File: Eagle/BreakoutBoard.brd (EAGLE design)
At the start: 77 x 30 mm, 17 parts, among them J1 JOINTS_CON, J2 RPI_CTRL, J3 RPI_PWR, J4 I2C_CTRL

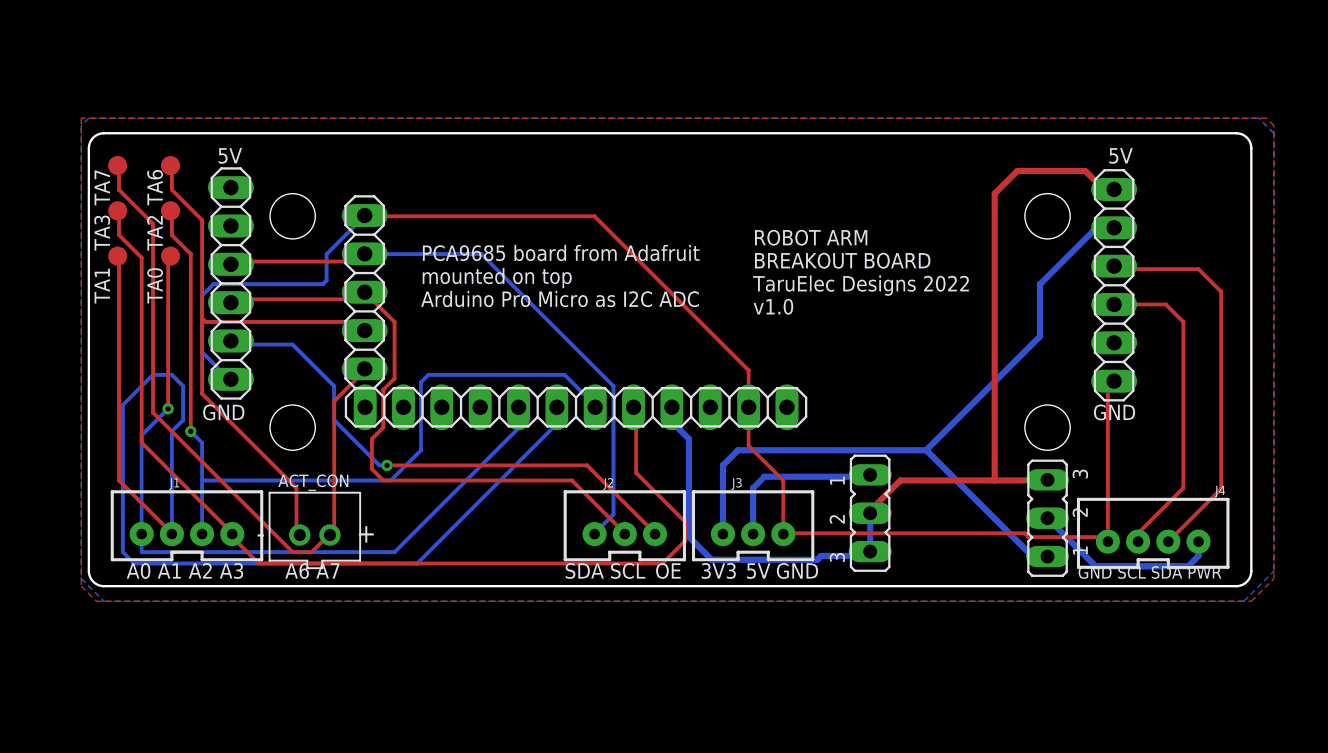
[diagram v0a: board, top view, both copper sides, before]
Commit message: Done some refactoring and readjusting
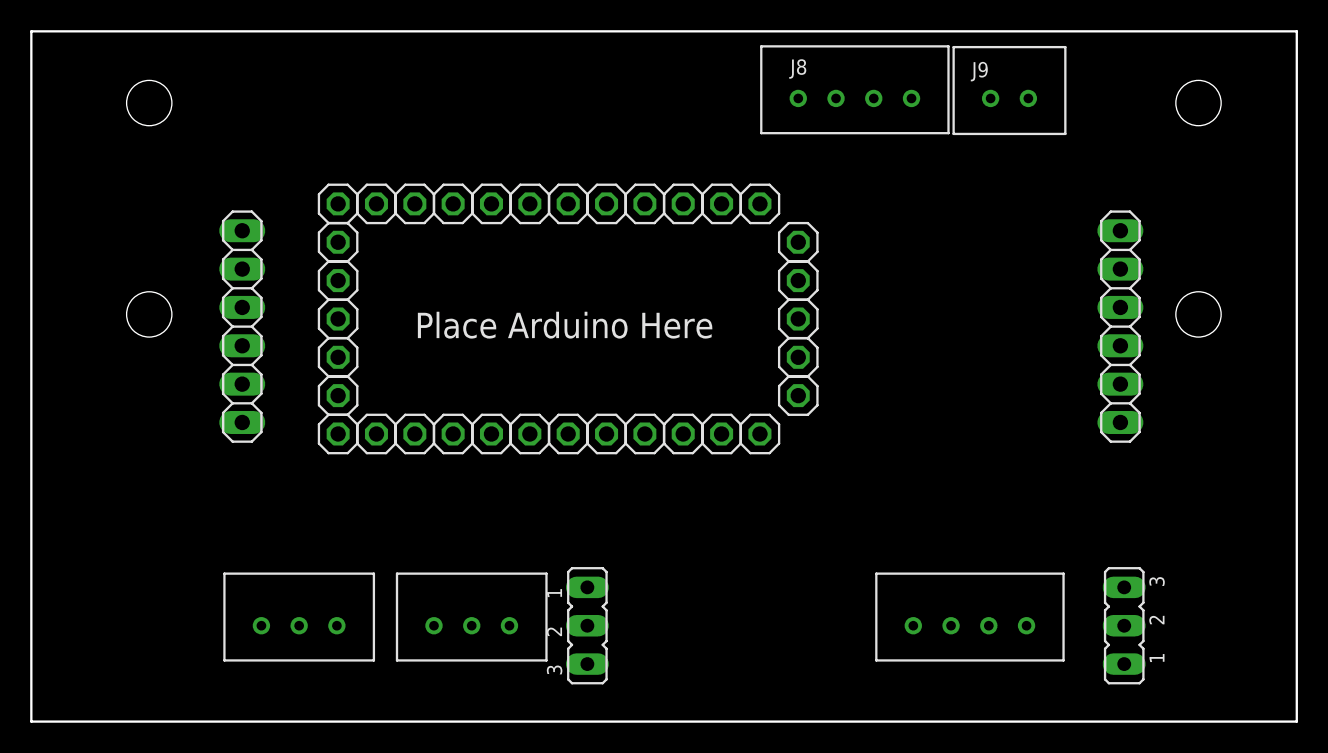
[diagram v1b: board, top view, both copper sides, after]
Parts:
- removed ACT_CON: (no value), adafruit:JST-PH-2-THM
- removed J1: JOINTS_CON, SparkFun-Connectors:JST-4-PTH-VERT
- removed J2: RPI_CTRL, SparkFun-Connectors:JST-3-PTH-VERT
- removed J3: RPI_PWR, SparkFun-Connectors:JST-3-PTH-VERT
- removed J4: I2C_CTRL, SparkFun-Connectors:JST-4-PTH-VERT
- removed TA0, TA1, TA2, TA3, TA6, TA7: TPB1,27, testpad:B1,27
- added J5: RPIDATA, Connector:B3B-XH-A
- added J6: RPIPWR, Connector:B3B-XH-A
- added J7: I2C, Connector:B4B-XH-A
- added J8: JOINTS1234, Connector:B4B-XH-A
- added J9: JOINTS56, Connector:B2B-XH-A
- added JP10: SDA, Connector:1X01
- added JP11, JP21, JP30, JP34: GND, Connector:1X01
- added JP12: D10, Connector:1X01
- added JP13: D11, Connector:1X01
- added JP14: D12, Connector:1X01
- added JP15: D13, Connector:1X01
- added JP16: A0, Connector:1X01
- added JP17: A1, Connector:1X01
- added JP18: A2, Connector:1X01
- added JP19: A3, Connector:1X01
- added JP20: 5V, Connector:1X01
- added JP22: RAW, Connector:1X01
- added JP23: D8, Connector:1X01
- added JP24: D7, Connector:1X01
- added JP25: D6, Connector:1X01
- added JP26: D5, Connector:1X01
- added JP27: D4, Connector:1X01
- added JP28: D3, Connector:1X01
- added JP29: D2, Connector:1X01
- added JP31: RST, Connector:1X01
- added JP32: TRXI, Connector:1X01
- added JP33, JP37: TX0, Connector:1X01
- added JP35: A_VCC, Connector:1X01
- added JP36: RXI, Connector:1X01
- added JP38: DTR, Connector:1X01
- added JP6: A7, Connector:1X01
- added JP8: A6, Connector:1X01
- added JP9: SCL, Connector:1X01
- JP3: value ARD_LEFT -> D9; device pinhead:1X05 -> Connector:1X01
- JP7: value ARD_BOT -> RST; device pinhead:1X12 -> Connector:1X01
- moved JP5 20.2 mm to (33.0, -7.62)
- moved JP7 15.2 mm to (39.4, 20.3)
- moved JP4 8.75 mm to (68.6, -7.62)
- moved JP3 6.11 mm to (16.5, 20.3), turned to 0 degrees
- moved JP2 2.95 mm to (10.2, 12.2)
- moved JP1 2.77 mm to (68.3, 12.2)
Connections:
- new net DTR: JP38.1
- new net RXI: JP36.1
- new net TX0: JP37.1
- net 3V3: now also J6.3; no longer J3.1
- net 5V: now also JP20.1, JP35.1; no longer JP7.9
- net A0: now also J8.1, JP16.1; no longer J1.1, JP7.5, TA0.TP
- net A1: now also J8.2, JP17.1; no longer J1.2, JP7.6, TA1.TP
- net A2: now also J8.3, JP18.1; no longer J1.3, JP7.7, TA2.TP
- net A3: now also J8.4, JP19.1; no longer J1.4, JP7.8, TA3.TP
- net A6: now also J9.2, JP8.1; no longer ACT_CON.2, JP3.4, TA6.TP
- net A7: now also J9.1, JP6.1; no longer ACT_CON.1, JP3.5, TA7.TP
- net D10: now also JP12.1; no longer JP7.1
- net D11: now also JP13.1; no longer JP7.2
- net D12: now also JP14.1; no longer JP7.3
- net D13: now also JP15.1; no longer JP7.4
- net GND: now also J6.1, J7.4, JP11.1, JP21.1, JP30.1, JP34.1; no longer J3.3, J4.1, JP3.1, JP7.11
- net I2CPWR: now also J7.1; no longer J4.4
- net OE: now also J5.1; no longer J2.3
- net RAW: now also JP22.1; no longer JP7.12
- net RPI5V: now also J6.2; no longer J3.2
- net RST: now also JP7.1; no longer JP7.10
- net SCL: now also J5.2, J7.3, JP9.1; no longer J2.2, J4.2, JP3.3
- net SDA: now also J5.3, J7.2, JP10.1; no longer J2.1, J4.3, JP3.2
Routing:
- net GND: track 94.5 -> 0.00 mm
- net A1: track 78.9 -> 0.00 mm
- net A3: track 66.4 -> 0.00 mm
- net SDA: track 65.9 -> 0.00 mm
- net 5V: track 65.3 -> 0.00 mm
- net SCL: track 62.0 -> 0.00 mm
- net A2: track 54.8 -> 0.00 mm, vias 1 -> 0
- net A0: track 50.2 -> 0.00 mm, vias 1 -> 0
- net 3V3: track 50.0 -> 0.00 mm
- net A7: track 45.3 -> 0.00 mm
- net A6: track 39.2 -> 0.00 mm
- net OE: track 34.8 -> 0.00 mm, vias 1 -> 0
- net I2CPWR: track 12.6 -> 0.00 mm
- net RPI5V: track 11.2 -> 0.00 mm
- removed copper zone on layer 1, net GND
- removed copper zone on layer 16, net GND
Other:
- board size 77 x 30 mm -> 83.8 x 45.7 mm
- board text added: "NC"
- board text added: "Place Arduino Here"
- board text added: "RPI5V"
- board text added: "VCC"
- board text removed: "A0 A1 A2 A3"
- board text removed: "A6 A7"
- board text removed: "GND SCL SDA PWR"
- board text removed: "PCA9685 board from Adafruit mounted on top Arduino Pro Micro as I2C ADC"
- board text removed: "ROBOT ARM BREAKOUT BOARD TaruElec Designs 2022 v1.0"
